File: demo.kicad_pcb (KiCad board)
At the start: 2 copper layers, 110 x 100 mm, 29 parts, among them J1 Conn_01x02, J2 Conn_01x04

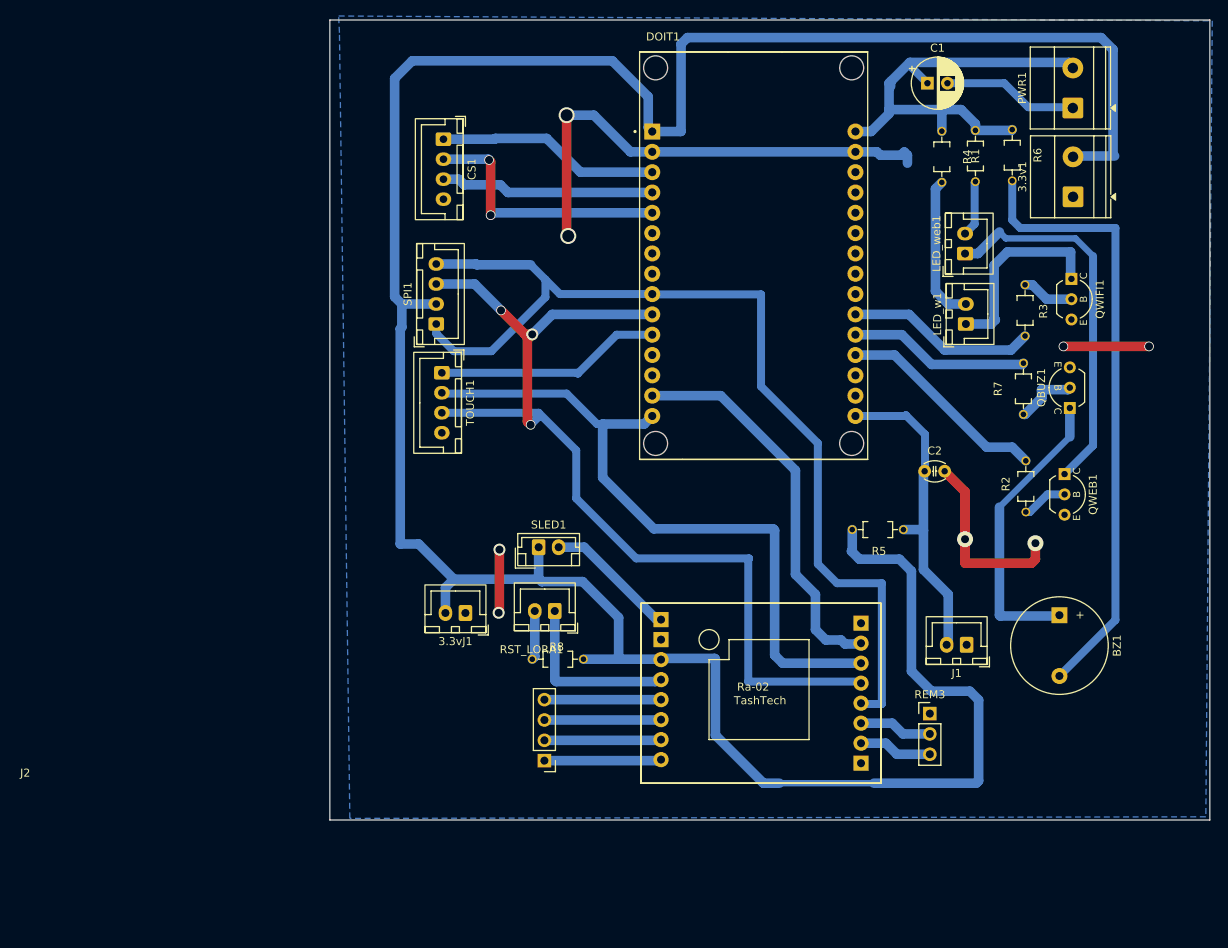
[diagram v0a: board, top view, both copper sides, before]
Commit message: latest update
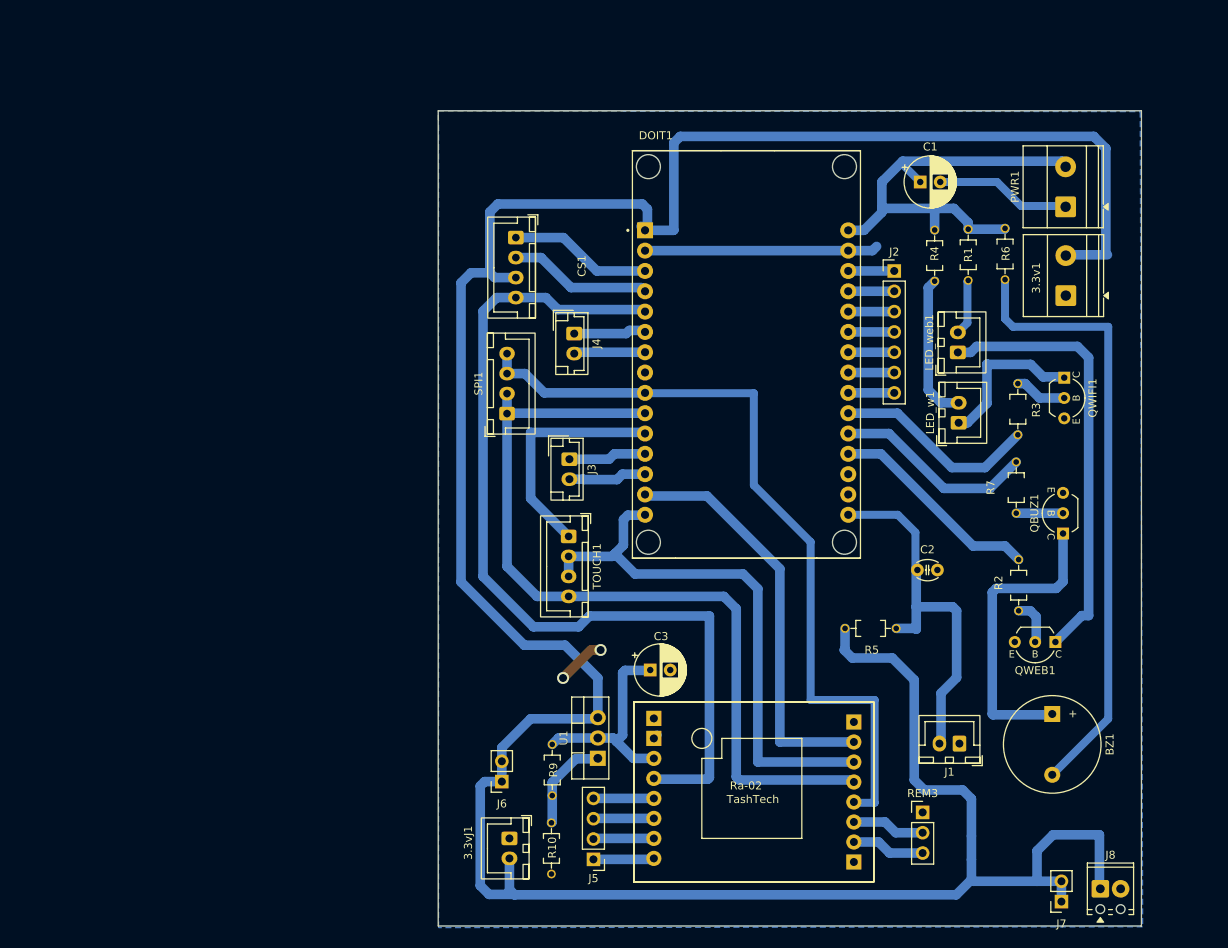
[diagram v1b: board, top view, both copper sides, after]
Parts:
- removed R8: 1K, LR0204F2K2:RESAD640W45L370D200
- removed RST_LORA1: Conn_01x02, Connector_JST:JST_XH_B2B-XH-A_1x02_P2.50mm_Vertical
- removed SLED1: Conn_01x02, Connector_JST:JST_EH_B2B-EH-A_1x02_P2.50mm_Vertical
- added C3: CP_Radial_D6.3mm_P2.50mm, PCM_Capacitor_THT_AKL:CP_Radial_D6.3mm_P2.50mm, F.Cu at (142.6, 121.2)
- added J3: JST_02, Connector_JST:JST_EH_B2B-EH-A_1x02_P2.50mm_Vertical, F.Cu at (132.4, 94.9)
- added J4: JST_02, Connector_JST:JST_EH_B2B-EH-A_1x02_P2.50mm_Vertical, F.Cu at (133.1, 79.2)
- added J5: Conn_01x04, Connector_PinHeader_2.54mm:PinHeader_1x04_P2.54mm_Vertical, F.Cu at (135.4, 144.9)
- added J6: PINHD_1x2_Female, Connector_PinSocket_2.54mm:PinSocket_1x02_P2.54mm_Vertical, F.Cu at (124.0, 135.2)
- added J7: PINHD_1x2_Female, Connector_PinSocket_2.54mm:PinSocket_1x02_P2.54mm_Vertical, F.Cu at (193.9, 150.2)
- added J8: PINHD_1x2_Female, TerminalBlock_Phoenix:TerminalBlock_Phoenix_MPT-0,5-2-2.54_1x02_P2.54mm_Horizontal, F.Cu at (198.8, 148.6)
- added R10: 10k, LR0204F2K2:RESAD640W45L370D200, F.Cu at (130.2, 143.6)
- added R9: 220, LR0204F2K2:RESAD640W45L370D200, F.Cu at (130.3, 133.8)
- added U1: LM317T, PCM_Package_TO_SOT_THT_AKL:TO-220-3_Vertical, F.Cu at (136.0, 132.3)
- J2: value Conn_01x04 -> JST_07; footprint Connector_PinHeader_2.54mm:PinHeader_1x04_P2.54mm_Vertical -> Connector_PinHeader_2.54mm:PinHeader_1x07_P2.54mm_Vertical
- moved J2 75.2 mm to (173.1, 71.4), turned to 0 degrees
- moved 3.3vJ1 28.7 mm to (125.0, 142.3), turned to -90 degrees
- moved TOUCH1 25.9 mm to (132.3, 104.5)
- moved QWEB1 21.0 mm to (193.2, 117.8), turned to 180 degrees
- moved QBUZ1 15.7 mm to (194.2, 104.2)
- moved CS1 15.3 mm to (125.8, 67.2)
- moved SPI1 14.3 mm to (124.7, 89.2)
- moved DOIT1 12.4 mm to (154.6, 81.8)
- moved R2 12.4 mm to (188.6, 110.7)
- moved R3 12.4 mm to (188.5, 88.7)
- moved R7 12.4 mm to (188.3, 98.5)
- moved REM3 12.4 mm to (176.6, 139.1)
- moved RF1 12.4 mm to (155.5, 138.3)
- moved 3.3v1 12.4 mm to (194.5, 74.5)
- moved C1 12.4 mm to (176.3, 60.2)
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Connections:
- CS1 pad 2: /RST -> /DC
- CS1 pad 3: /DC -> +3.3V
- CS1 pad 4: /MOSI -> /RST
- DOIT1 pad 22: unconnected-(DOIT1-D33-Pad22) -> /D33
- DOIT1 pad 23: unconnected-(DOIT1-D25-Pad23) -> /D25
- DOIT1 pad 24: unconnected-(DOIT1-D26-Pad24) -> /D26
- DOIT1 pad 25: unconnected-(DOIT1-D27-Pad25) -> /D27
- DOIT1 pad 26: unconnected-(DOIT1-D14-Pad26) -> /D14
- DOIT1 pad 27: unconnected-(DOIT1-D12-Pad27) -> /D12
- DOIT1 pad 28: unconnected-(DOIT1-D13-Pad28) -> /D13
- J2 pad 1: Net-(J2-Pin_1) -> /D13
- J2 pad 2: Net-(J2-Pin_2) -> /D12
- J2 pad 3: Net-(J2-Pin_3) -> /D14
- J2 pad 4: Net-(J2-Pin_4) -> /D27
- REM3 pad 1: unconnected-(REM3-Pin_1-Pad1) -> GND
- RF1 pad 3: +3.3V -> Net-(RF1-3.3V)
- RF1 pad 4: /RST_LORA -> /RST
- RF1 pad 5: Net-(J2-Pin_4) -> Net-(J5-Pin_4)
- RF1 pad 6: Net-(J2-Pin_3) -> Net-(J5-Pin_3)
- RF1 pad 7: Net-(J2-Pin_2) -> Net-(J5-Pin_2)
- RF1 pad 8: Net-(J2-Pin_1) -> Net-(J5-Pin_1)
- RF1 pad 9: unconnected-(RF1-GND-Pad9) -> GND
- SPI1 pad 1: /SCK -> /MISO
- SPI1 pad 2: +3.3V -> /MISO
- SPI1 pad 3: /MISO -> /SCK
- TOUCH1 pad 3: /MISO -> /MOSI
- TOUCH1 pad 4: /TIRQ -> /MISO
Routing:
- net GND: track 136.9 -> 52.8 mm, vias 8 -> 2
- net /RST: track 33.0 -> 113.6 mm, vias 2 -> 0
- net +3.3V: track 340.2 -> 368.9 mm
- net /SCK: track 126.9 -> 99.1 mm
- net Net-(RF1-3.3V): track 0.00 -> 27.1 mm
- net /RST_LORA: track 21.7 -> 0.00 mm
- net /MISO: track 123.4 -> 106.2 mm, vias 3 -> 0
- net /MOSI: track 85.7 -> 69.5 mm
- net Net-(J2-Pin_1): track 14.3 -> 0.00 mm
- net Net-(J2-Pin_2): track 14.2 -> 0.00 mm
- net Net-(J2-Pin_3): track 14.2 -> 0.00 mm
- net Net-(J2-Pin_4): track 14.2 -> 0.00 mm
- net Net-(R10-Pad1): track 0.00 -> 12.0 mm
- net /TX0: track 0.00 -> 9.75 mm
- net /RX0: track 0.00 -> 9.73 mm
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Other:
- board size 110 x 100 mm -> 87.9 x 101.9 mm
